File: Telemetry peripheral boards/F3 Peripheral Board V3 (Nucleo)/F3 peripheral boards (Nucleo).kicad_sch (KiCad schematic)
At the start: 47 parts, among them J1 ATS668LSM, J2 Exit Connector, J3 Potentiometer, J4 Strain Gauge, J5 Tire temp Sensor, U1 LM2907M/NOPB, U2 INA125U, U3 MCP2515-I/SO, U4 ISO1050DUB, U5 ATtiny1616-S, U6 LM7805CV, U7 LF33CV, Y1 STDCSU1-8M

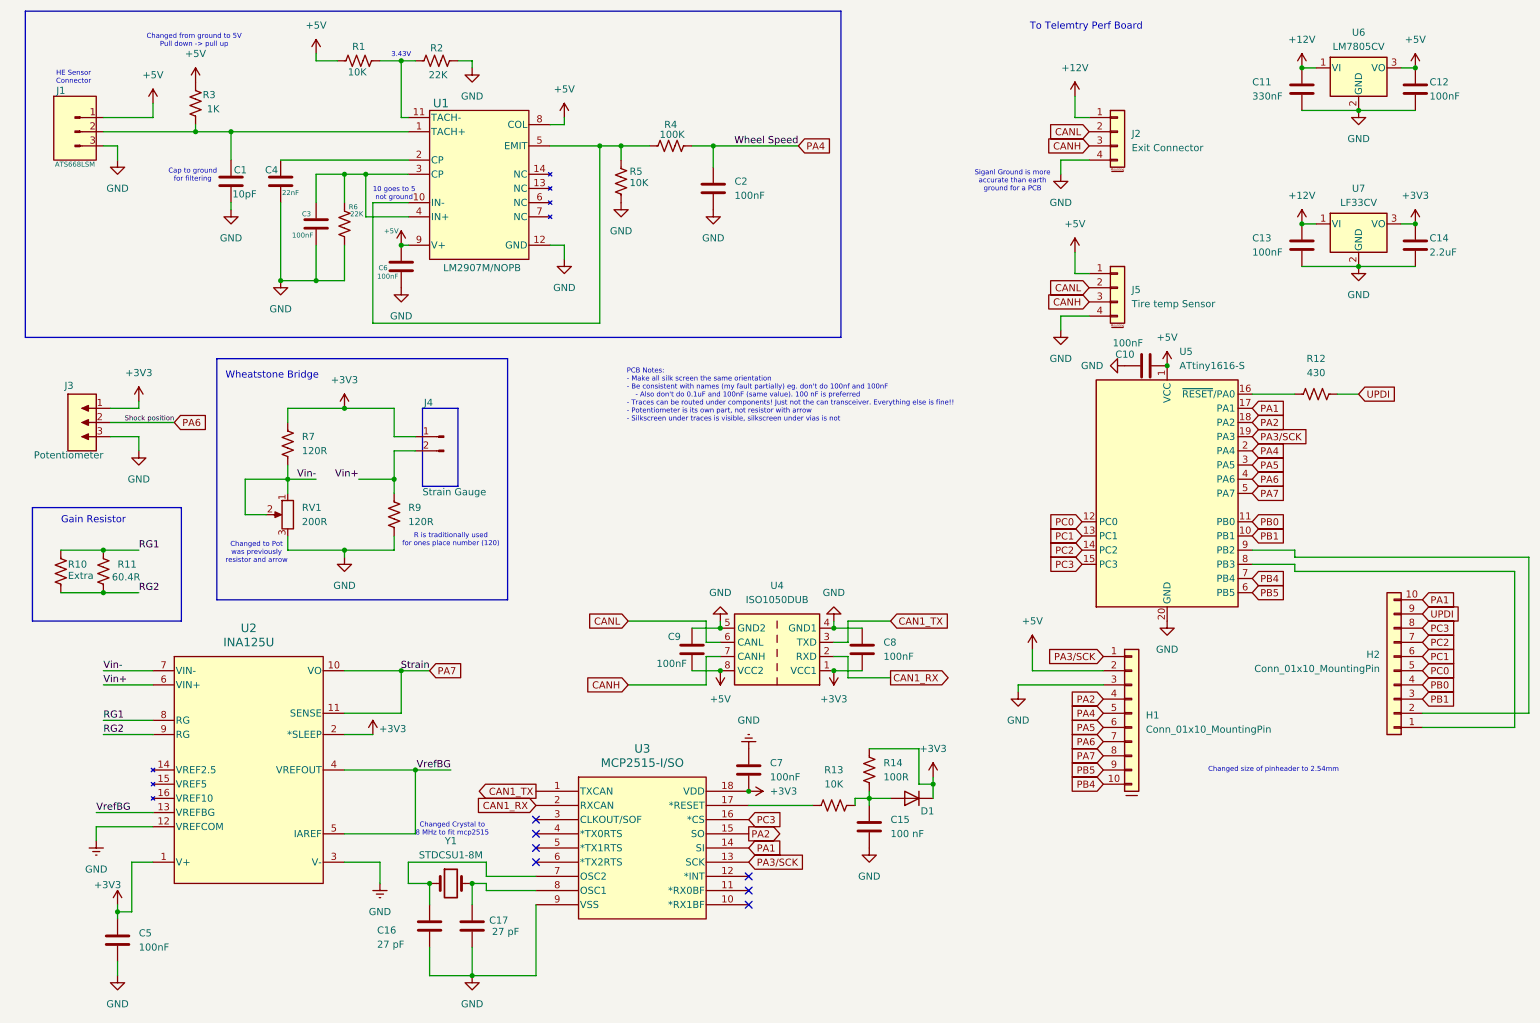
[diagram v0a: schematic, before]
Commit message: updated schematic and pcb new components
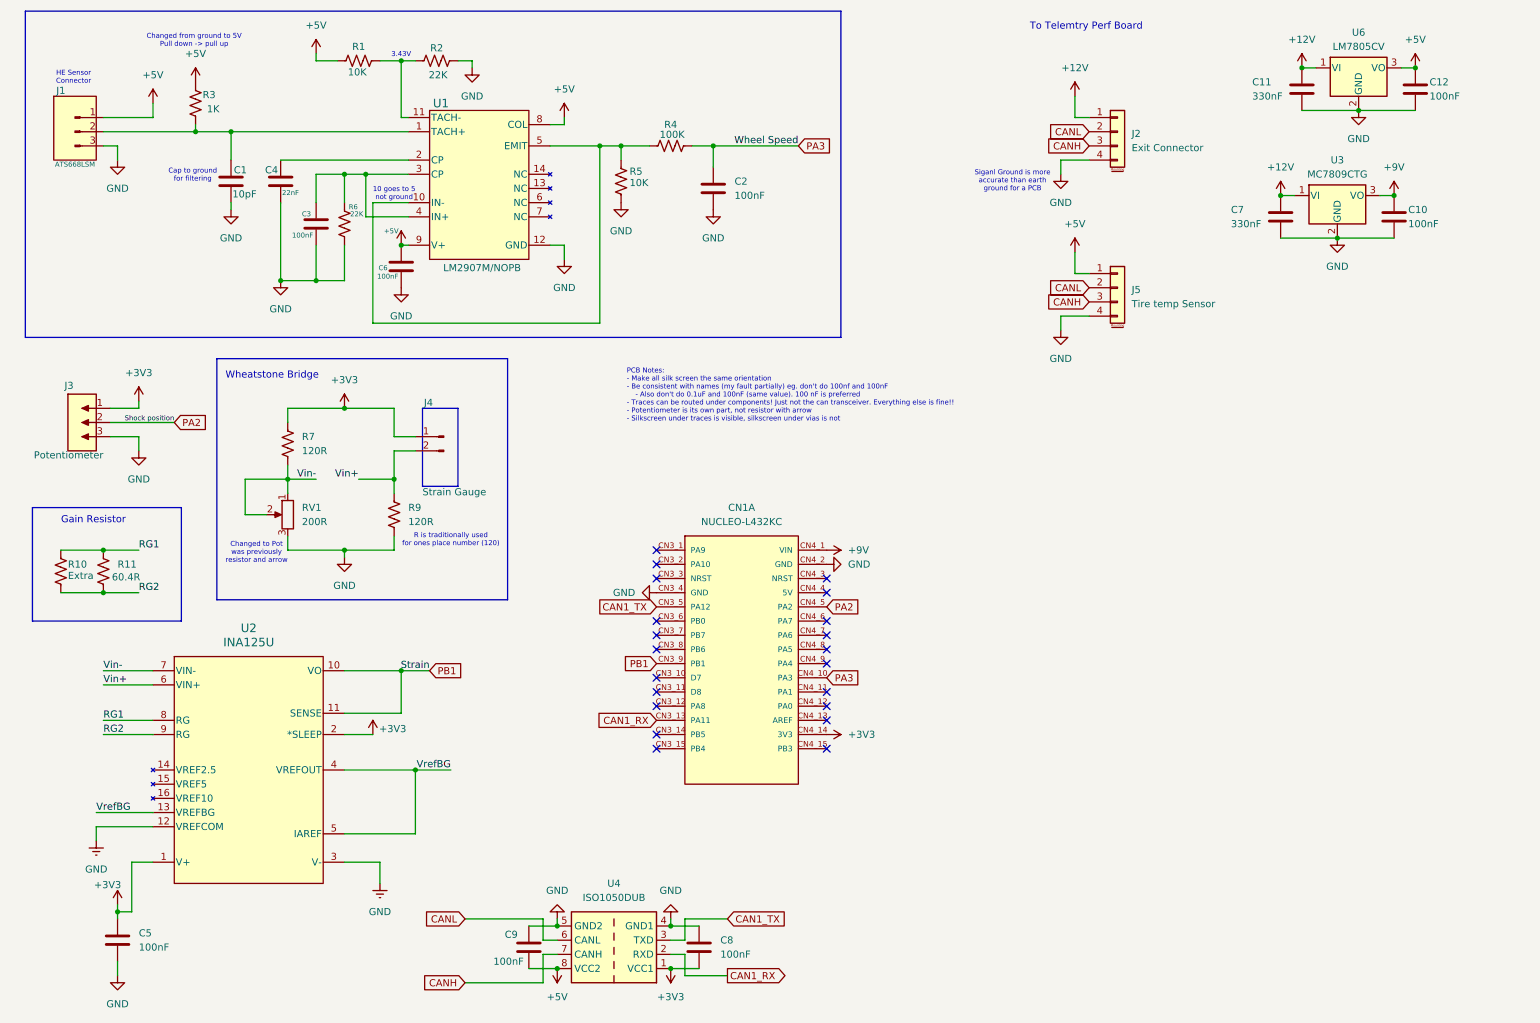
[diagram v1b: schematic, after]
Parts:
- removed C13: 100nF, Capacitor_SMD:C_0805_2012Metric_Pad1.18x1.45mm_HandSolder, symbol Device:C
- removed C14: 2.2uF, Capacitor_SMD:C_0805_2012Metric_Pad1.18x1.45mm_HandSolder, symbol Device:C
- removed C15: 100 nF, Capacitor_SMD:C_0805_2012Metric_Pad1.18x1.45mm_HandSolder, symbol Device:C
- removed C16, C17: 27 pF, Capacitor_SMD:C_0805_2012Metric_Pad1.18x1.45mm_HandSolder, symbol Device:C
- removed D1: D, Diode_SMD:D_0805_2012Metric, symbol Device:D
- removed H1, H2: Conn_01x10_MountingPin, Connector_PinHeader_2.54mm:PinHeader_1x10_P2.54mm_Vertical, symbol Connector_Generic_MountingPin:Conn_01x10_MountingPin
- removed R12: 430, Resistor_SMD:R_0805_2012Metric_Pad1.20x1.40mm_HandSolder, symbol Device:R_US
- removed R13: 10K, Resistor_SMD:R_0805_2012Metric_Pad1.20x1.40mm_HandSolder, symbol Device:R_US
- removed R14: 100R, Resistor_SMD:R_0805_2012Metric_Pad1.20x1.40mm_HandSolder, symbol Device:R_US
- removed U3: MCP2515-I/SO, Package_SO:SOIC-18W_7.5x11.6mm_P1.27mm, symbol FS_3_Global_Symbol_Library:MCP2515-I_SO
- removed U5: ATtiny1616-S, Package_SO:SOIC-20W_7.5x12.8mm_P1.27mm, symbol MCU_Microchip_ATtiny:ATtiny1616-S
- removed U7: LF33CV, Package_TO_SOT_THT:TO-220-3_Vertical, symbol Regulator_Linear:LM7805_TO220
- removed Y1: STDCSU1-8M, Crystal:Crystal_SMD_5032-2Pin_5.0x3.2mm_HandSoldering, symbol Device:Crystal
- added CN1: NUCLEO-L432KC, FS_3_Global_Footprint_Library:NUCLEO-L432KC, symbol FS3_Global_Symbol_Library:NUCLEO-L432KC
- added U3: MC7809CTG, Package_TO_SOT_THT:TO-220-3_Vertical, symbol Regulator_Linear:LM7805_TO220
- C7: value 100nF -> 330nF
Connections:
- net PA6 is gone; now on net PA2: J3.2
- net PA7 is gone; now on net PB1: U2.10 (VO), U2.11 (SENSE)
- net +12V: now also C7.1, U3.1 (VI)
- net +3V3: now also CN1.CN4_14 (3V3); no longer C7.2
- net +5V: no longer C10.2
- net CAN1_RX: now also CN1.CN3_13 (PA11)
- net GND: now also C10.2, C7.2, CN1.CN3_4 (GND), CN1.CN4_2 (GND), U3.2 (GND); no longer C10.1, C7.1
- net PA2: now also CN1.CN4_5 (PA2)
- net PB1: now also CN1.CN3_9 (PB1)
- net PA4 renamed PA3
- net PA3: now also CN1.CN4_10 (PA3)
- new net +9V: C10.1, CN1.CN4_1 (VIN), U3.3 (VO)
- no-connect marks 7 -> 21
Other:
- note removed: "Changed Crystal to 8 MHz to fit mcp2515"
- note removed: "Changed size of pinheader to 2.54mm"
- moved on the sheet: C8, C9, U4

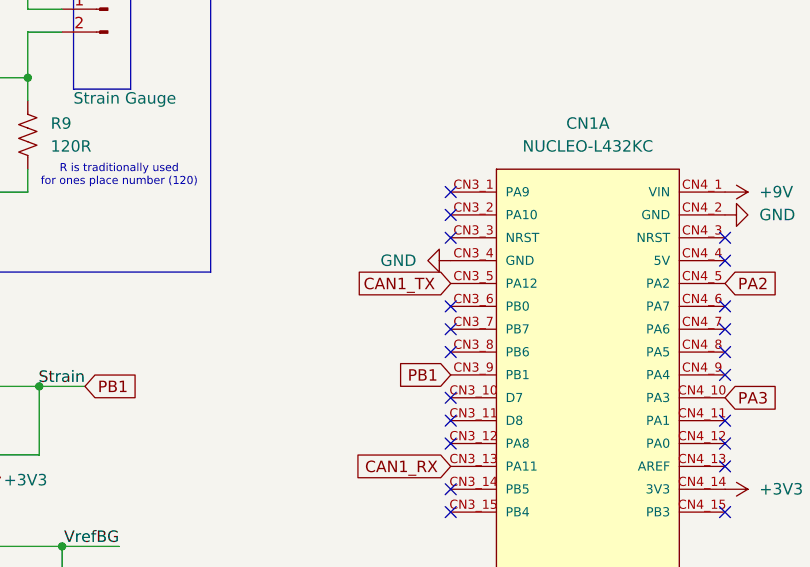
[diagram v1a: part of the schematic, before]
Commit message: PCB (Partially Complete)
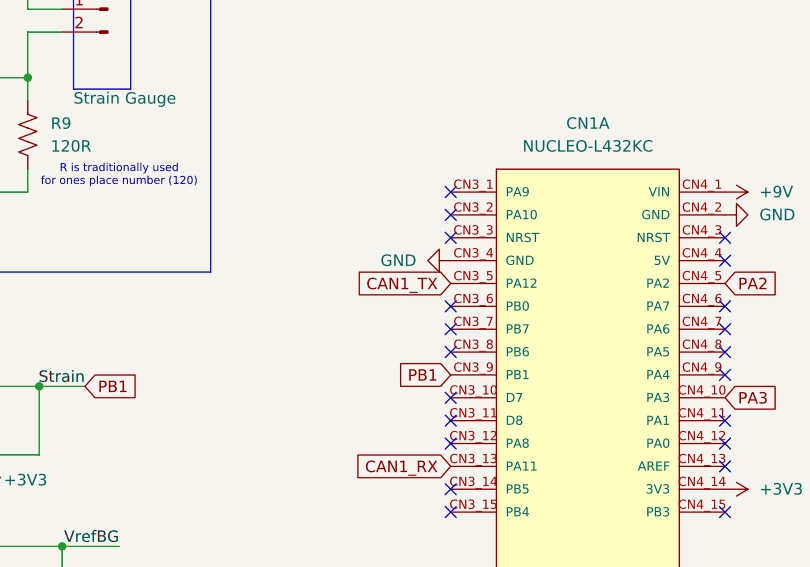
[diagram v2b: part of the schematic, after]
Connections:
- net CAN1_TX: now also CN1.CN3_5 (PA12)
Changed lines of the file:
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@@
-		)
-	)
-	(global_label "CAN1_TX"
-		(shape output)
-		(at 116.84 120.65 0)
-		(fields_autoplaced yes)
-		(effects
-			(font
-				(size 1.27 1.27)
-			)
-			(justify left)
-		)
-		(property "Intersheetrefs" "${INTERSHEET_REFS}"
-			(at 127.8685 120.65 0)
-			(effects
-				(font
-					(size 1.27 1.27)
-				)
-				(justify left)
-				(hide yes)
-			)
 		)
 	)
@@
 			(effects
 				(font
+					(size 1.27 1.27)
+				)
+				(justify right)
+				(hide yes)
+			)
+		)
+	)
+	(global_label "CAN1_TX"
+		(shape input)
+		(at 127 120.65 180)
+		(fields_autoplaced yes)
+		(effects
+			(font
+				(size 1.27 1.27)
+			)
+			(justify right)
+		)
+		(property "Intersheetrefs" "${INTERSHEET_REFS}"
+			(at 115.9715 120.65 0)
+			(effects
+				(font

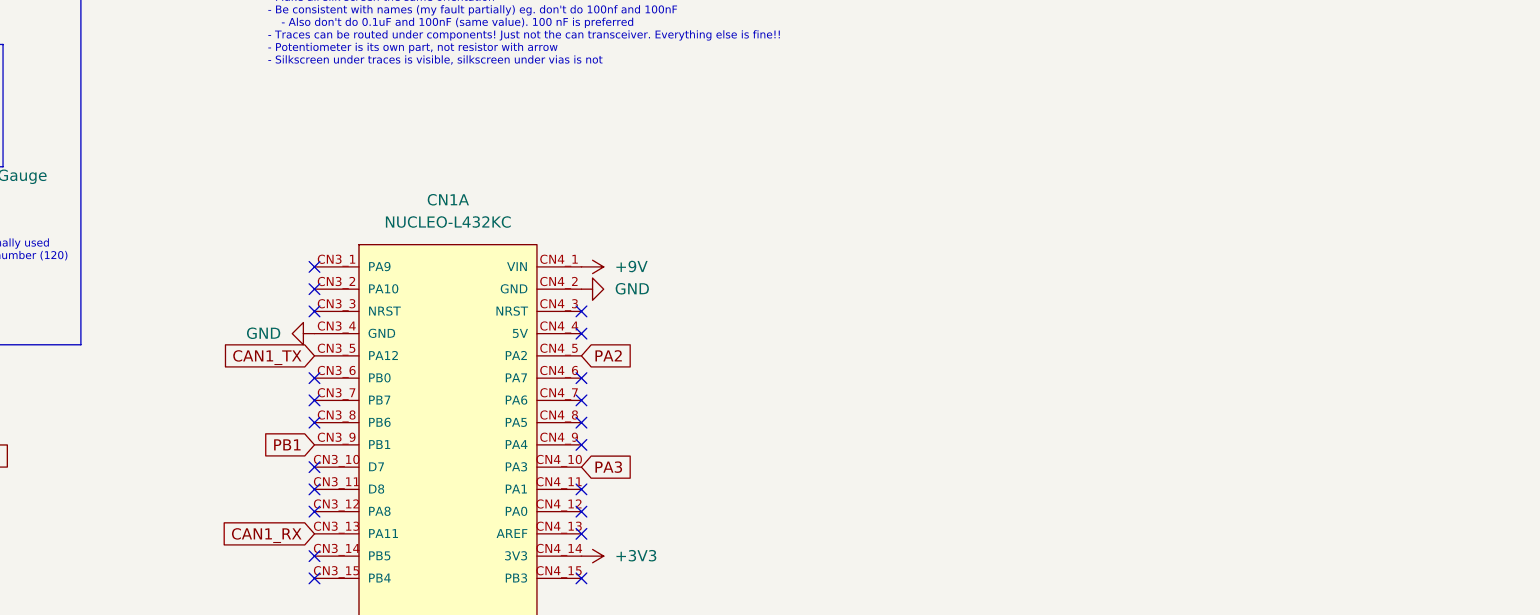
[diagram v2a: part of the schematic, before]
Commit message: Update F3 peripheral boards (Nucleo).kicad_sch
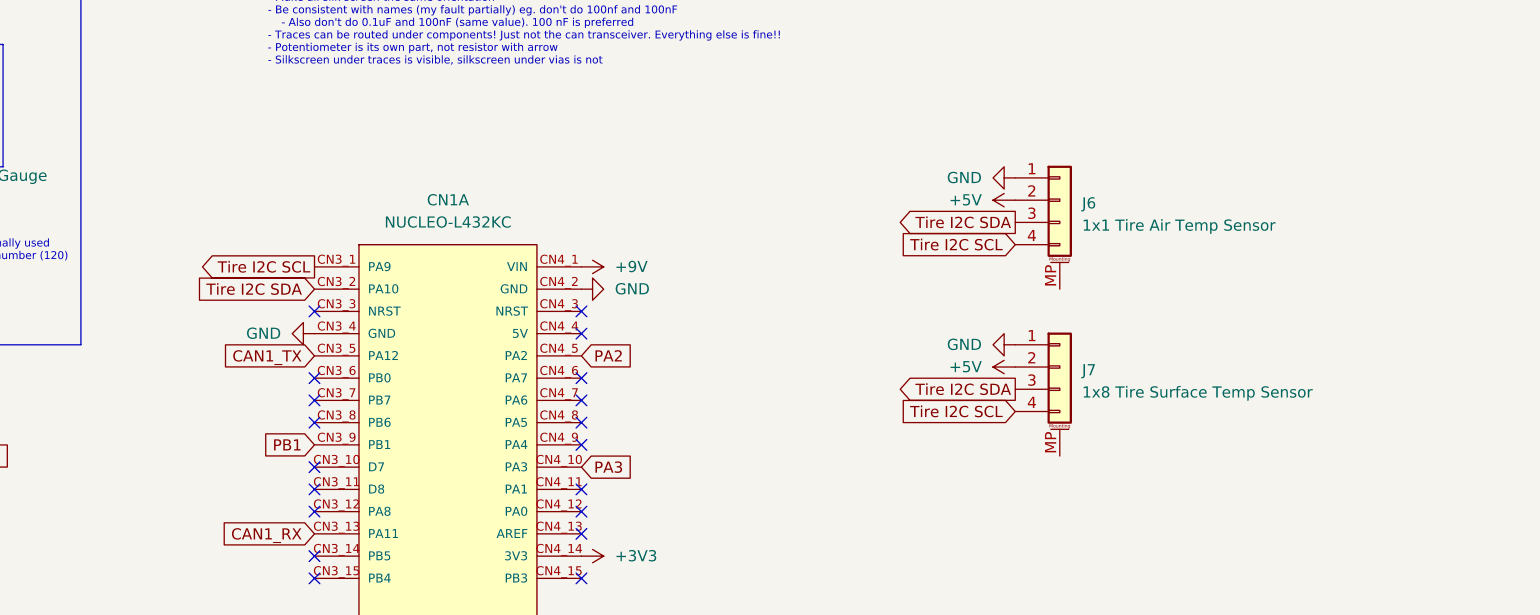
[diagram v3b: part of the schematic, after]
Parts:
- added J6: 1x1 Tire Air Temp Sensor, Connector_Molex:Molex_Nano-Fit_105309-xx04_1x04_P2.50mm_Vertical, symbol Connector_Generic_MountingPin:Conn_01x04_MountingPin
- added J7: 1x8 Tire Surface Temp Sensor, Connector_Molex:Molex_Nano-Fit_105309-xx04_1x04_P2.50mm_Vertical, symbol Connector_Generic_MountingPin:Conn_01x04_MountingPin
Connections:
- net +5V: now also J6.2 (Pin_2), J7.2 (Pin_2)
- net GND: now also J6.1 (Pin_1), J7.1 (Pin_1)
- net Tire I2C SCL: now reaches CN1.CN3_1 (PA9)
- net Tire I2C SCL: now also J6.4 (Pin_4), J7.4 (Pin_4)
- net Tire I2C SDA: now reaches CN1.CN3_2 (PA10)
- net Tire I2C SDA: now also J6.3 (Pin_3), J7.3 (Pin_3)
- no-connect marks 21 -> 19
